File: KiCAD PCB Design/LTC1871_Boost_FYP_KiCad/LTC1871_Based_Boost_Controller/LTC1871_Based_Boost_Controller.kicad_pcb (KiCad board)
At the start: 2 copper layers, 60 x 80 mm, 29 parts, among them J2 J2_OUT, Q1 IRF7811, U1 LTC1871EMS-7-PBF

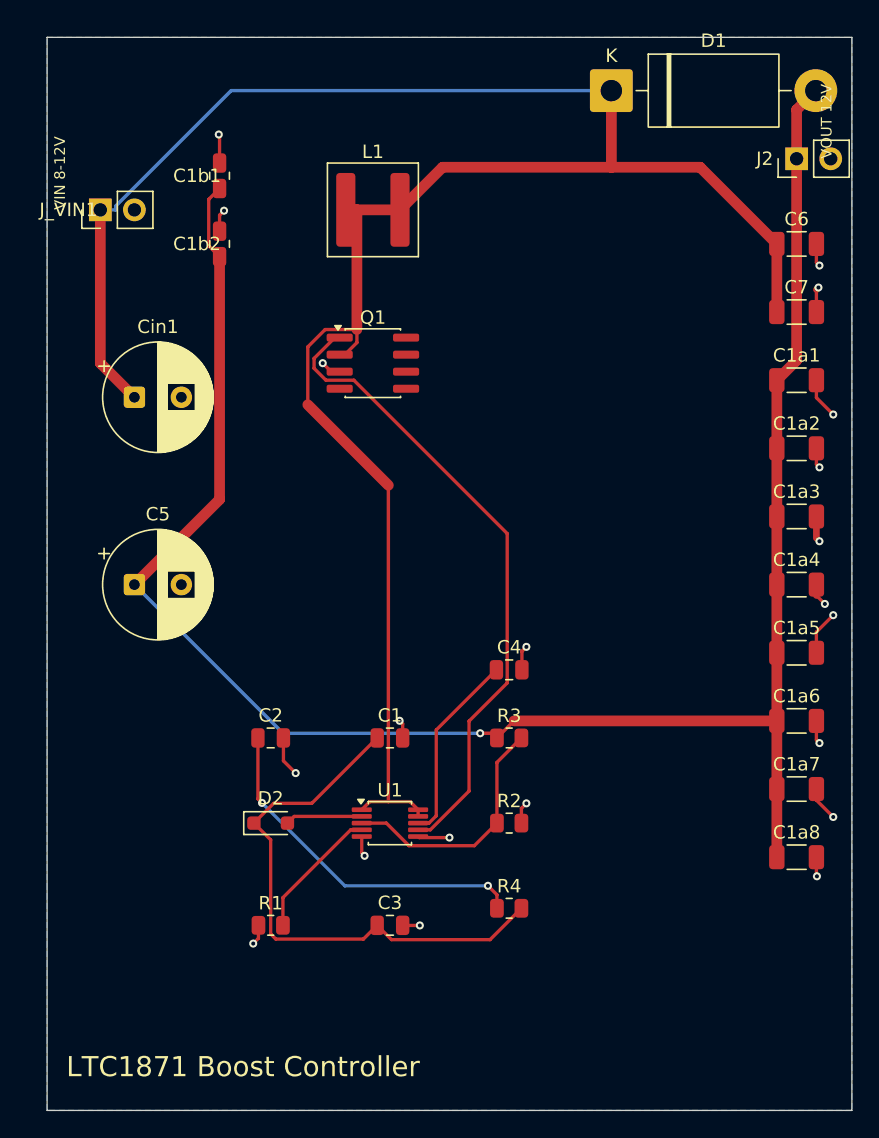
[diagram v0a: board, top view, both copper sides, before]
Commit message: Auto-sync from Fortune at 2026-04-08 23:49:32
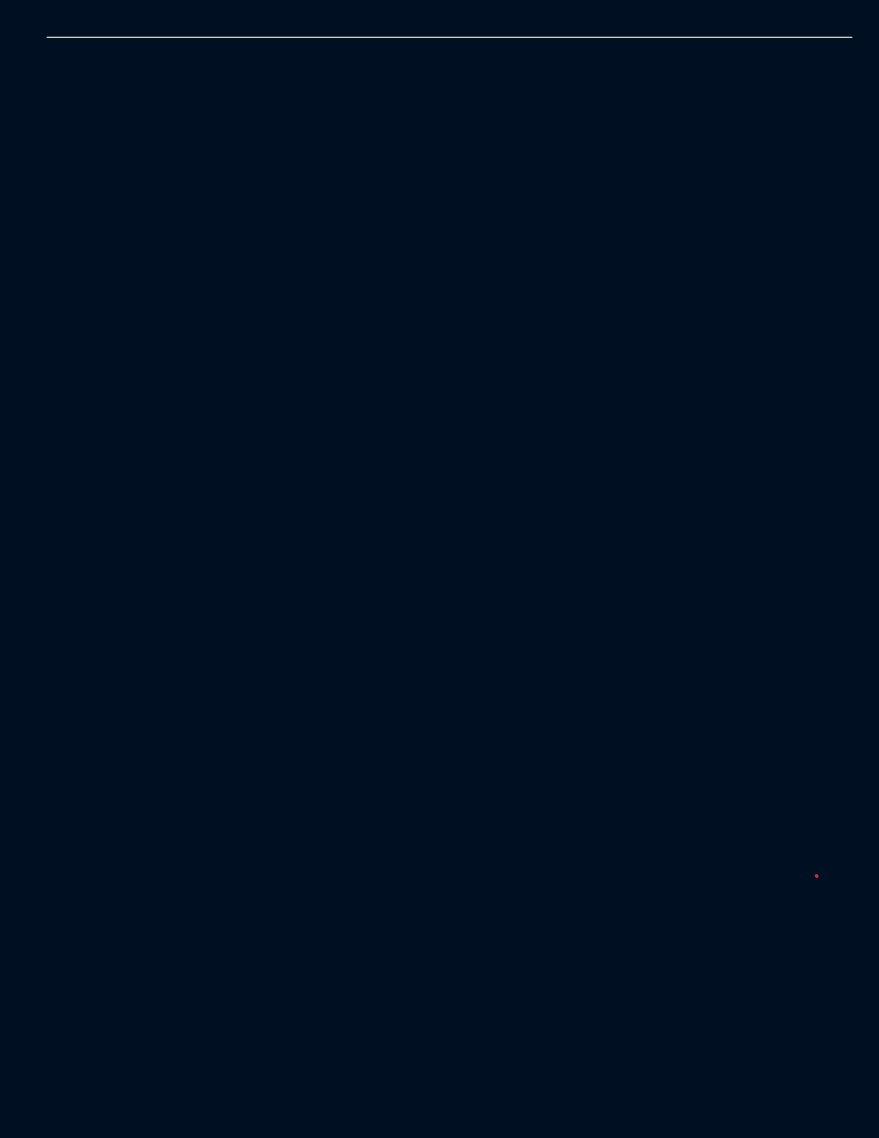
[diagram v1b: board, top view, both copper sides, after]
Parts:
- removed C1: 10n, Capacitor_SMD:C_0805_2012Metric
- removed C1a1, C1a2, C1a3, C1a4, C1a5, C1a6, C1a7, C1a8, C6, C7: 22µ, Capacitor_SMD:C_1206_3216Metric
- removed C1b1, C1b2: 10µ, Capacitor_SMD:C_0805_2012Metric
- removed C2: 6.8n, Capacitor_SMD:C_0805_2012Metric
- removed C3: 100p, Capacitor_SMD:C_0805_2012Metric
- removed C4: 4.7µ, Capacitor_SMD:C_0805_2012Metric
- removed C5, Cin1: 100µ, Capacitor_THT:CP_Radial_D8.0mm_P3.50mm
- removed D1: MBR735, Diode_THT:D_DO-201AD_P15.24mm_Horizontal
- removed D2: 1N4148, Diode_SMD:D_SOD-323_HandSoldering
- removed J2: J2_OUT, Connector_PinHeader_2.54mm:PinHeader_1x02_P2.54mm_Vertical
- removed J_VIN1: J_VIN_OUT, Connector_PinHeader_2.54mm:PinHeader_1x02_P2.54mm_Vertical
- removed L1: 10µ, Inductor_SMD:L_Coilcraft_XAL6060-XXX
- removed Q1: IRF7811, Package_SO:SOIC-8_3.9x4.9mm_P1.27mm
- removed R1: 68.1k, Resistor_SMD:R_0805_2012Metric
- removed R2: 56k, Resistor_SMD:R_0805_2012Metric
- removed R3: 499k, Resistor_SMD:R_0805_2012Metric
- removed R4: 8.66k, Resistor_SMD:R_0805_2012Metric
- removed U1: LTC1871EMS-7-PBF, Package_SO:MSOP-10_3x3mm_P0.5mm
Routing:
- net Net-(D1-K): track 160.9 -> 0.00 mm
- net Net-(D1-A): track 144.3 -> 0.00 mm, vias 1 -> 0
- net Net-(Q1-G): track 48.2 -> 0.00 mm
- net Net-(D2-K): track 41.3 -> 0.00 mm
- net GND: track 40.8 -> 0.06 mm, vias 21 -> 0
- net Net-(C2-Pad1): track 26.3 -> 0.00 mm, vias 2 -> 0
- net Net-(U1-FB): track 18.6 -> 0.00 mm
- net Net-(U1-INTVCC): track 14.3 -> 0.00 mm
- net Net-(U1-FREQ): track 10.0 -> 0.00 mm
- net Net-(D2-A): track 5.75 -> 0.00 mm
- removed copper zone on B.Cu, net GND
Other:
- board outline removed
- board text removed: "LTC1871 Boost Controller"
- board text removed: "VIN 8-12V"
- board text removed: "VOUT 12V"
